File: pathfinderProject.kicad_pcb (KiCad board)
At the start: 2 copper layers, 10 parts, among them SW1 SW_Push, SW2 SW_Push, SW3 SW_Push, U1 XIAO-RP2040-DIP

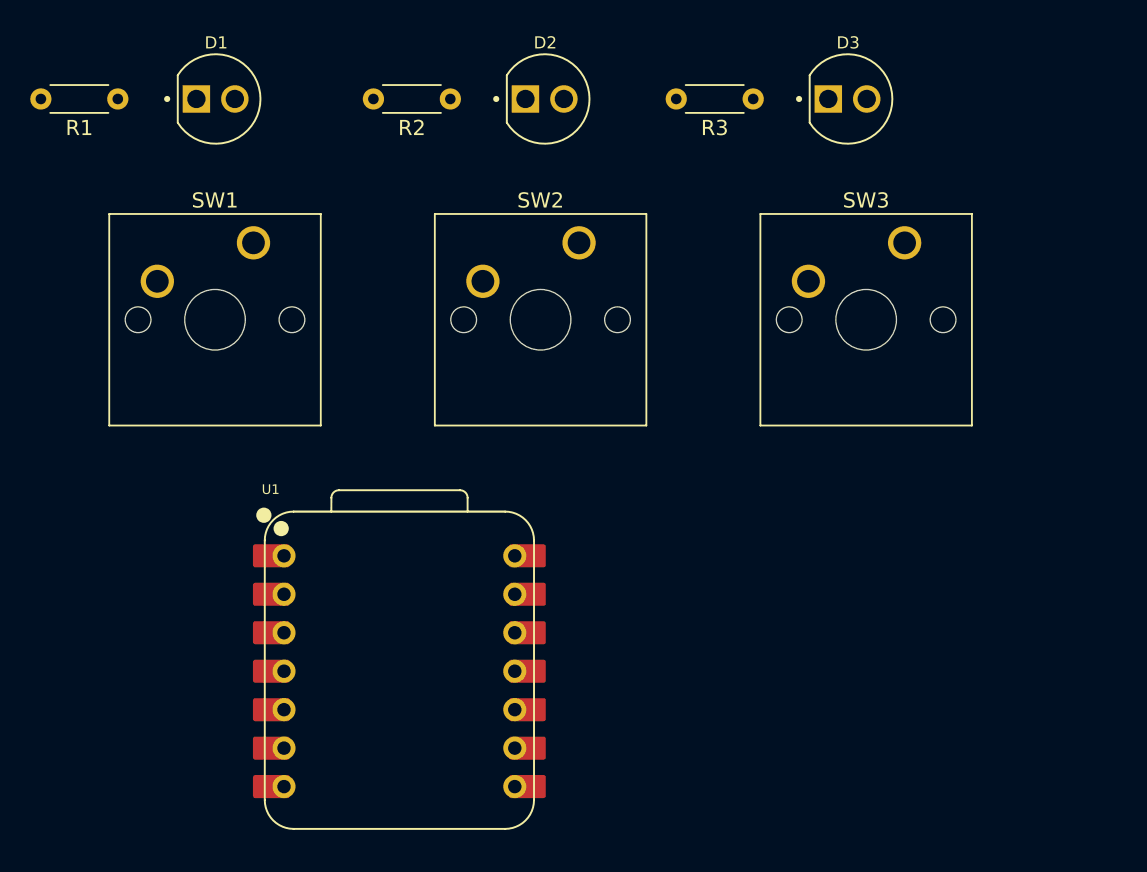
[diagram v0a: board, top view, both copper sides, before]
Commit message: Add files via upload
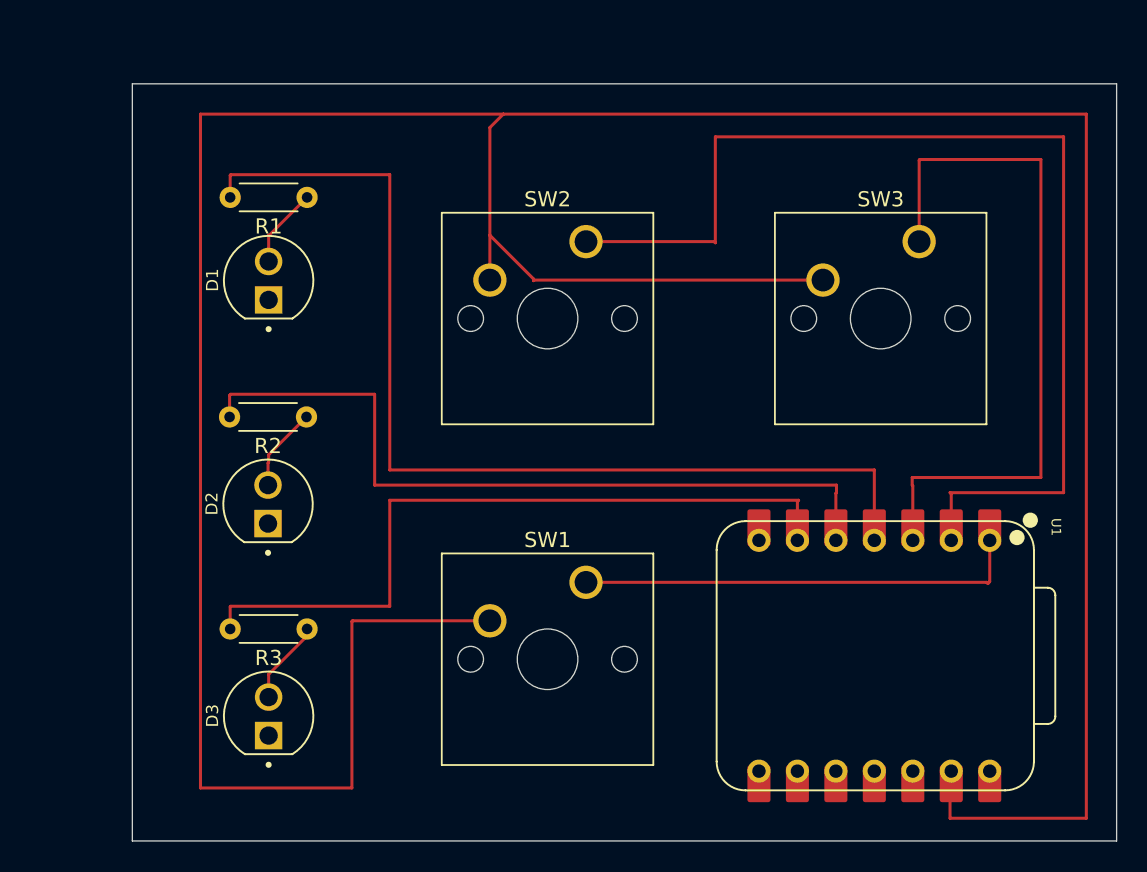
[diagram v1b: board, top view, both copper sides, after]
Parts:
- moved D3 55.9 mm to (134.0, 71.8), turned to 90 degrees
- moved R3 45.7 mm to (136.5, 66.0)
- moved D2 32.4 mm to (134.0, 57.8), turned to 90 degrees
- moved SW1 31.4 mm to (155.0, 62.9)
- moved U1 31.4 mm to (174.0, 67.8), turned to -90 degrees
- moved R2 23.0 mm to (136.5, 52.0)
- moved R1 14.1 mm to (136.5, 37.5)
- moved D1 12.5 mm to (134.0, 43.0), turned to 90 degrees
- moved SW3 0.96 mm to (177.0, 40.4)
- moved SW2 0.47 mm to (155.0, 40.4)
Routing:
- net GND: track 0.00 -> 226.4 mm
- net button2: track 0.00 -> 72.8 mm
- net LED1: track 0.00 -> 68.2 mm
- net LED2: track 0.00 -> 51.2 mm
- net LED3: track 0.00 -> 48.7 mm
- net button3: track 0.00 -> 47.1 mm
- net button1: track 0.00 -> 29.5 mm
- net Net-(D2-PadA): track 0.00 -> 5.55 mm
- net Net-(D3-PadA): track 0.00 -> 5.55 mm
- net Net-(D1-PadA): track 0.00 -> 5.31 mm
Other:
- board outline added: 65 x 50 mm
